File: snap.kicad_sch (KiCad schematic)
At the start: 95 parts, among them J1 Conn_02x07_Odd_Even, Q1 CSD25310Q2, Q10 DMG1012T, Q11 DMG1012T, Q7 DMG1012T, Q8 DMG1012T, Q9 DMG1012T, SW3 SW_DPST, SW4 SW_DPST, U1 BG95-MF, U2 SGM2036S-ADJXN5G/TR, U3 STM32H7B3VITx, U4 SGM2036S-ADJXN5G/TR, U5 TXS0108EPW, Y3 8kHz, Y4 32.768kHz

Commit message: time to lock in for the schematic!!! (continued)
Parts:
- added C46, C47, C48: 33pF, symbol Device:C
- added C49, C53, C54, C55, C56: 100nF, symbol Device:C
- added C50: 1nF, symbol Device:C
- added C51, C52: 10nF, symbol Device:C
- added D8: TPD5E003DPFR, Package_SON:WSON-6-1EP_2x2mm_P0.65mm_EP1x1.6mm, symbol TPD5E003DPFR:TPD5E003DPFR
- added J2: JAE_SIM_Card_SF72S006, Connector_JAE:JAE_SIM_Card_SF72S006, symbol Connector:JAE_SIM_Card_SF72S006
- added J3: DF12NB(3.0)-36DS-0.5V(51), symbol Connector_Generic_MountingPin:Conn_02x18_Odd_Even_MountingPin
- added J4: Micro_SD_Card_Det_Hirose_DM3AT, Connector_Card:microSD_HC_Hirose_DM3AT-SF-PEJM5, symbol Connector:Micro_SD_Card_Det_Hirose_DM3AT
- added Q12, Q13, Q3, Q4, Q5, Q6: DTC143ZE3, symbol Transistor_BJT:DTC143Z
- added Q2: 2SC4617TLQ, symbol Device:Q_NPN
- added R24, R25, R26: 0R, symbol Device:R_Small
- added R27: 15K, symbol Device:R_Small
- added R28: 51K, symbol Device:R_Small
- added R29, R30: 4.7K, symbol Device:R
- added R31: 1K, symbol Device:R
- added R32, R33, R34, R37: 10K, symbol Device:R
- added R35, R36: 51K, symbol Device:R
- added R38: 120K, symbol Device:R
- added R39: 100K, symbol Device:R
- added U6: SN74AVC2T245RSWR, Package_DFN_QFN:UQFN-10_1.4x1.8mm_P0.4mm, symbol SN74AVC2T245RSWR:SN74AVC2T245RSWR
- AE1: value 1575AT43A0040001E -> 0830AT54A2200001E
- D6, D7: value LED -> HB-CLM3A-BKW-GKW
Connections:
- net ANTENNA_3V: now also C28.1, C29.1, C30.1, R5.1, U2.5 (VOUT); no longer C16.1, C17.1, C18.1, R1.1, U4.5 (VOUT)
- net ANT_GNSS: now also U1.49 (ANT_GNSS)
- net ANT_MAIN: now also U1.60 (ANT_MAIN)
- net AP_READY_MCU: now also Q2.E
- net GND: now also U1.100 (GND), U1.101 (GND), U1.102 (GND), U1.3 (GND), U1.31 (GND), U1.47 (USIM_GND), U1.48 (GND), U1.50 (GND), U1.54 (GND), U1.55 (GND), U1.58 (GND), U1.59 (GND), U1.61 (GND), U1.62 (GND), U1.67 (GND), U1.68 (GND), U1.69 (GND), U1.70 (GND), U1.71 (GND), U1.72 (GND), U1.73 (GND), U1.74 (GND), U1.79 (GND), U1.80 (GND), U1.81 (GND), U1.82 (GND), U1.89 (GND), U1.90 (GND), U1.91 (GND), U5.11 (GND), C46.2, C47.2, C48.2, C49.2, C51.2, C52.2, C53.2, C54.2, C55.2, C56.2, D8.2 (A), J2.C5 (GND), J2.CSW, J2.SH, Q12.2 (E), Q13.2 (E), Q3.2 (E), Q4.2 (E), Q5.2 (E), Q6.2 (E), R35.2, R36.1, R38.1, U6.10 (1DIR), U6.3 (GND), U6.9 (GND)
- net GNSS_EN_MCU: now also R32.2
- net GNSS_RXD_MCU: now also U6.9 (GND)
- net GNSS_TXD_MCU: now also U6.8 (A1)
- net LED_R: no longer R17.2, R19.2, R21.2
- net MAIN_CTS_MCU: now also U1.36 (MAIN_CTS), U5.13 (B7)
- net MAIN_DCD_MCU: now also U1.38 (MAIN_DCD), U5.17 (B3)
- net MAIN_DTR_MCU: now also U1.30 (MAIN_DTR), U5.14 (B6)
- net MAIN_RI_MCU: now also U1.39 (MAIN_RI), U5.18 (B2)
- net MAIN_RTS_MCU: now also U1.37 (MAIN_RTS), U5.16 (B4)
- net MAIN_RXD_MCU: now also U1.34 (MAIN_RXD), U5.12 (B8)
- net MAIN_TXD_MCU: now also U1.35 (MAIN_TXD), U5.15 (B5)
- net NET_STATUS: now also U1.21 (NET_STATUS)
- net PON_TRIG_1V8: now also C16.1, C17.1, C18.1, R1.1, U4.5 (VOUT); no longer C28.1, C29.1, C30.1, R5.1, U2.5 (VOUT)
- net PON_TRIG_MCU: now also R39.2
- net PSM_IND_MCU: now also Q12.3 (C), R33.2
- net PWRKEY_MCU: now also Q4.1 (B)
- net RESET_MCU: now also Q5.1 (B)
- net RF_GPIO_06: now also Q3.1 (B)
- net RF_GPIO_10: now also Q13.3 (C), R34.2
- net STATUS: now also U1.20 (STATUS), Q13.1 (B)
- net VBAT_BB: now also U1.32 (VBAT_BB), U1.33 (VBAT_BB)
- net VBAT_RF: now also U1.52 (VBAT_RF), U1.53 (VBAT_RF)
- net VDD_MCU: now also U5.19 (VCCB), C53.1, C56.1, R33.1, R34.1, U6.1 (2DIR), U6.7 (VCCA)
- net PSM_IND: now reaches U1.1 (PSM_IND)
- net PSM_IND: now also Q12.1 (B)
- net PWRKEY: now reaches U1.15 (PWRKEY)
- net PWRKEY: now also C52.1, Q4.3 (C)
- net RESET_N: now reaches U1.17 (~{RESET})
- net RESET_N: now also Q5.3 (C)
- net W_DISABLE#: now reaches U1.18 (GPIO5)
- net W_DISABLE#: now also C51.1, Q3.3 (C)
- net AP_READY: now reaches U1.19 (GPIO6)
- net AP_READY: now also Q2.C, R29.2
- net GNSS_TXD: now reaches U1.27 (GPIO11)
- net GNSS_TXD: now also U6.5 (B1)
- net GNSS_RXD: now reaches U1.28 (GPIO12)
- net GNSS_RXD: now also U6.4 (B2)
- net VDD_EXT: now reaches U1.29 (VDD_EXT)
- net VDD_EXT: now also U5.2 (VCCA), C50.1, C54.1, C55.1, R28.2, R29.1, R30.1, R37.2, U6.6 (VCCB)
- net USIM_DET: now reaches U1.42 (USIM_DET)
- net USIM_DET: now also D8.6 (K5), J2.DSW, R28.1
- net USIM_VDD_SOCKET: now reaches U1.43 (USIM_VDD)
- net USIM_VDD_SOCKET: now also C49.1, D8.1 (K1), J2.C1 (VCC), R27.1
- net USIM_RST_SOCKET: now reaches U1.44 (USIM_RST)
- net USIM_RST_SOCKET: now also R24.2
- net USIM_DATA_SOCKET: now reaches U1.45 (USIM_DATA)
- net USIM_DATA_SOCKET: now also R26.2
- net USIM_CLK_SOCKET: now reaches U1.46 (USIM_CLK)
- net USIM_CLK_SOCKET: now also R25.2
- net PON_TRIG: now reaches U1.96 (PON_TRIG)
- net PON_TRIG: now also R39.1
- net at U5.1 (A1): now also R35.1
- net at U5.10 (OE): now also R37.1, R38.2
- net at U5.20 (B1): now also R36.2
- net MAIN_RI: now reaches U5.3 (A2)
- net MAIN_DCD: now reaches U5.4 (A3)
- net MAIN_RTS: now reaches U5.5 (A4)
- net MAIN_RXD: now reaches U5.6 (A5)
- net MAIN_DTR: now reaches U5.7 (A6)
- net MAIN_CTS: now reaches U5.8 (A7)
- net MAIN_TXD: now reaches U5.9 (A8)
- new net: C46.1, D8.3 (K2), J2.C2 (RST), R24.1
- new net: C47.1, D8.4 (K3), J2.C3 (CLK), R25.1
- new net: C48.1, D8.5 (K4), J2.C7 (I/O), R26.1, R27.2
- new net: C50.2, Q2.B, R30.2
- new net: Q6.1 (B), R32.1
- new net EN: Q6.3 (C), R31.2, U6.2 (~{OE})
- new net RGB_LED_B: R17.2
- new net RGB_LED_G: R19.2
- new net RGB_LED_R: R21.2
- no-connect marks 6 -> 34
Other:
- moved on the sheet: C1, C10, C11, C12, C13, C14, C15, C16, C17, C18, C19, C2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

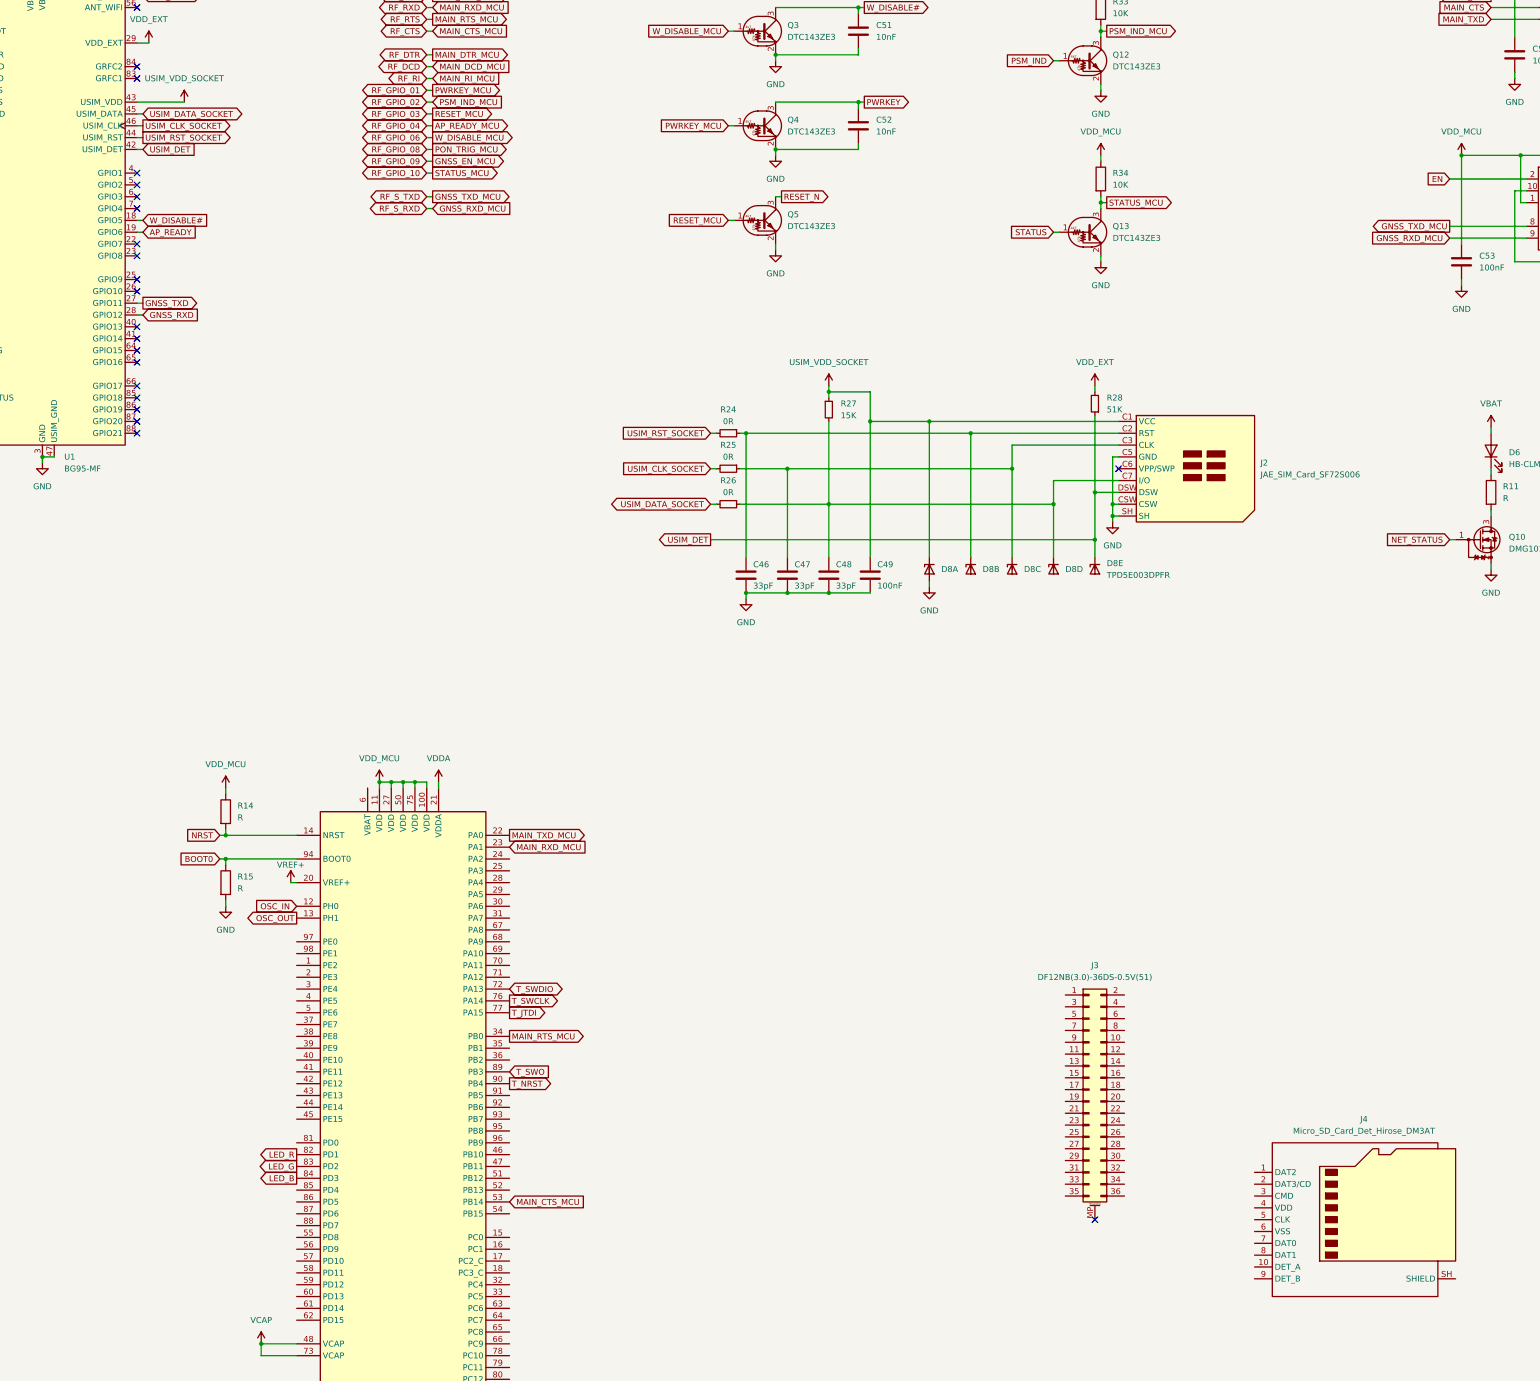
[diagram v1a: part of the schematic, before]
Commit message: time to lock in for the schematic!!! (continued)
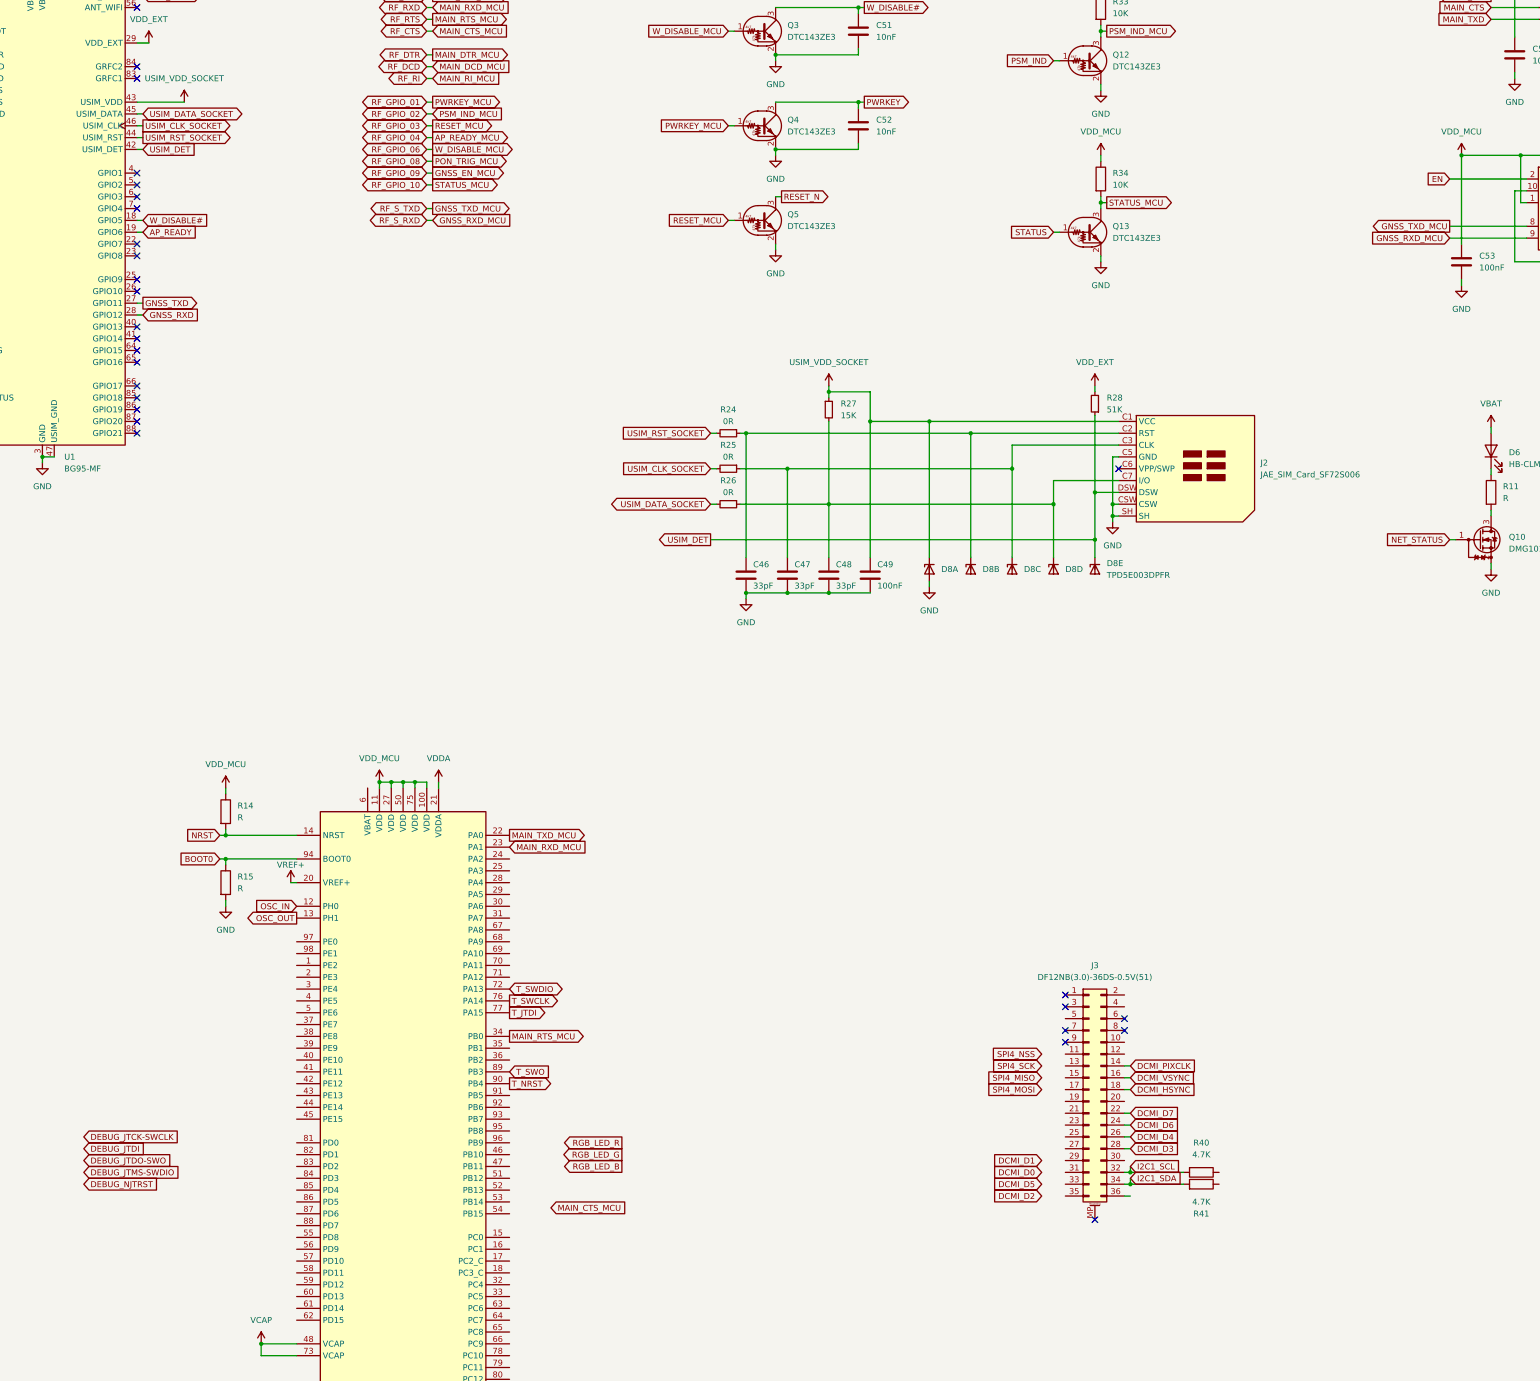
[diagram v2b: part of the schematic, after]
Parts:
- removed J4: Micro_SD_Card_Det_Hirose_DM3AT, Connector_Card:microSD_HC_Hirose_DM3AT-SF-PEJM5, symbol Connector:Micro_SD_Card_Det_Hirose_DM3AT
- added R40, R41: 4.7K, symbol Device:R
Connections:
- net MAIN_CTS_MCU: no longer U3.53 (PB14)
- net DCMI_PIXCLK: now reaches J3.14 (Pin_14)
- net DCMI_VSYNC: now reaches J3.16 (Pin_16)
- net DCMI_HSYNC: now reaches J3.18 (Pin_18)
- net DCMI_D7: now reaches J3.22 (Pin_22)
- net DCMI_D6: now reaches J3.24 (Pin_24)
- net DCMI_D4: now reaches J3.26 (Pin_26)
- net DCMI_D3: now reaches J3.28 (Pin_28)
- net I2C1_SCL: now reaches J3.32 (Pin_32)
- net I2C1_SCL: now also R40.2
- net I2C1_SDA: now reaches J3.34 (Pin_34)
- net I2C1_SDA: now also R41.2
- net LED_B: no longer names the net of U3.84 (PD3)
- net LED_G: no longer names the net of U3.83 (PD2)
- net LED_R: no longer names the net of U3.82 (PD1)
- no-connect marks 34 -> 40
